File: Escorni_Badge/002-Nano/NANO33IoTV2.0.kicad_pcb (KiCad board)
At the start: 4 copper layers, 99.5 x 97.2 mm, 1 part

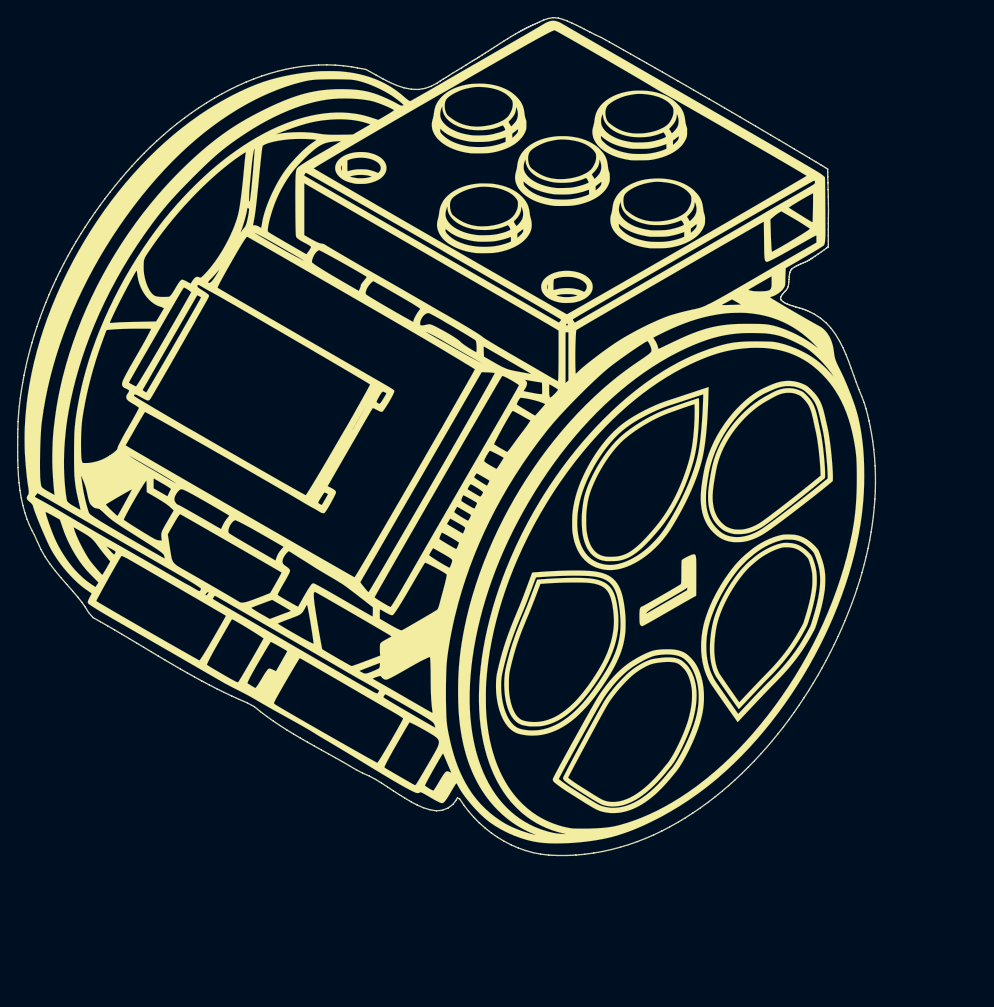
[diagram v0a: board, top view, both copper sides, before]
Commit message: Add some minors changes
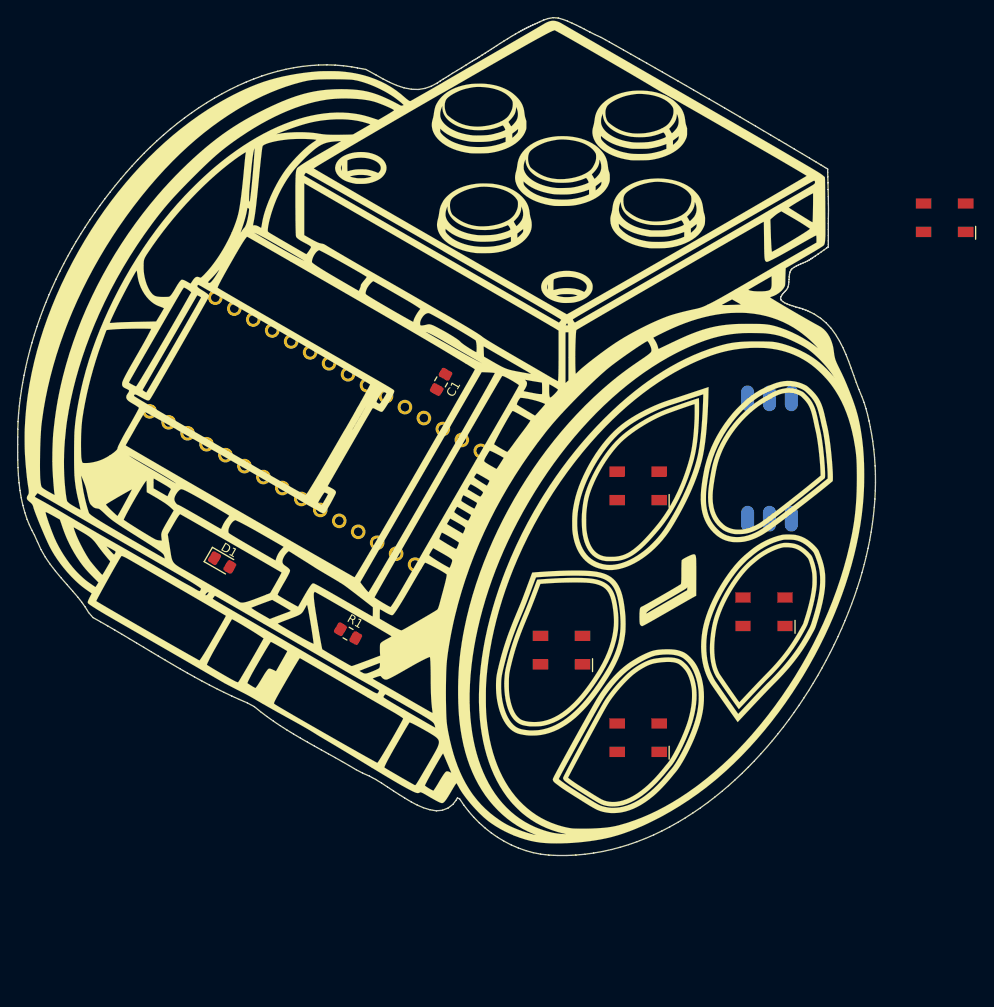
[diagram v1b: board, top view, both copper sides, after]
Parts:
- added C1: 22nF, Capacitor_SMD:C_0805_2012Metric_Pad1.15x1.40mm_HandSolder, F.Cu at (142.9, 97.8)
- added D1: LED, LED_SMD:LED_0805_2012Metric_Pad1.15x1.40mm_HandSolder, F.Cu at (117.5, 118.7)
- added J1: Arduino-NANO-33, Arduino:NANO_33_Single_Socket, F.Cu at (128.3, 103.5)
- added LED1: WS2812B, 002:WS2812B, F.Cu at (165.7, 109.9)
- added LED2: WS2812B, 002:WS2812B, F.Cu at (156.8, 128.9)
- added LED3: WS2812B, 002:WS2812B, F.Cu at (165.7, 139.1)
- added LED4: WS2812B, 002:WS2812B, F.Cu at (180.3, 124.5)
- added LED5: WS2812B, 002:WS2812B, F.Cu at (201.3, 78.7)
- added R1: 1k, Resistor_SMD:R_0805_2012Metric_Pad1.15x1.40mm_HandSolder, F.Cu at (132.1, 127.0)
- added REF**: WS2812B_Module, 002-Nano:WS2812B_Module, B.Cu at (181.0, 106.7)

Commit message: Updates
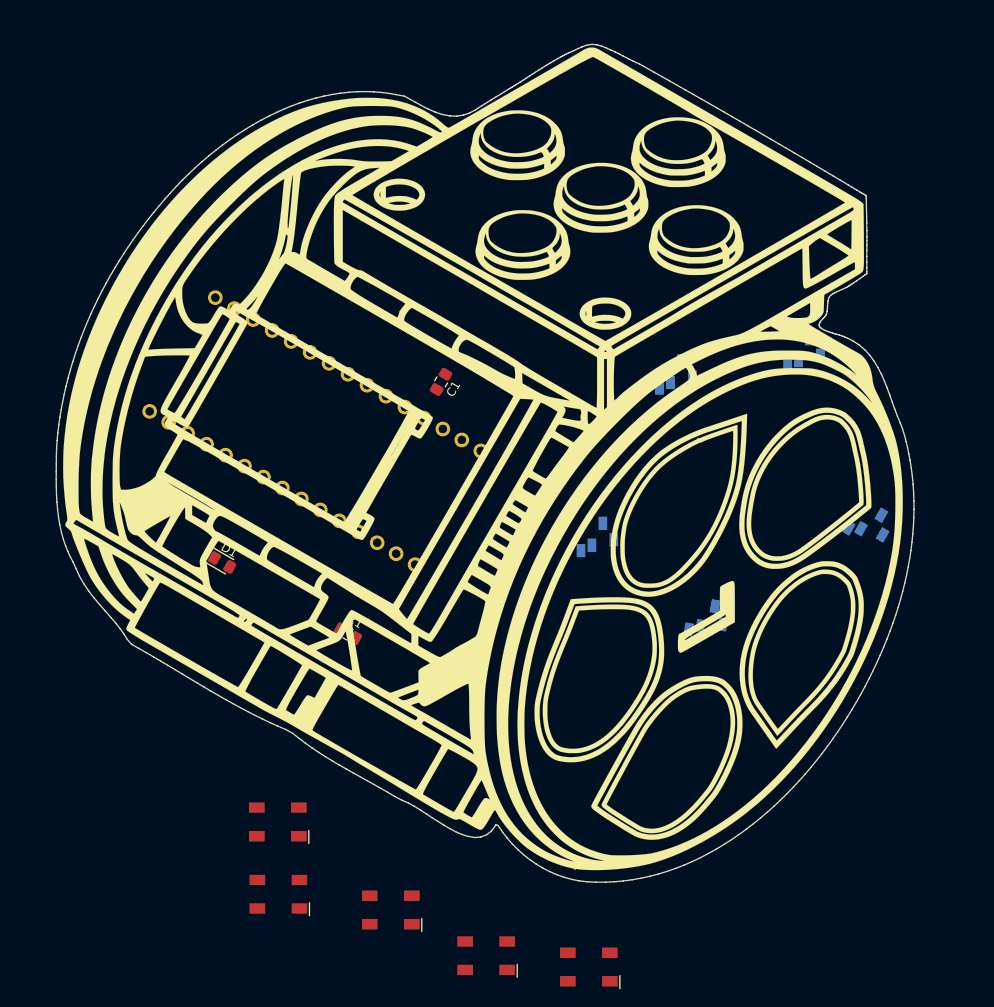
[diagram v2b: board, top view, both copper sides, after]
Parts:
- removed the REF** at (181.0, 106.7)
- removed SilKs1: Escorni_Art, 002-Nano:escorni-badge-new_05_Nano_100mm
- added REF**: P9823_Reverse_Mount_Short_Pin, 002-Nano:P9823_Reverse_Mount_Short_Pin, B.Cu at (172.6, 131.9)
- added REF**: P9823_Reverse_Mount_Short_Pin, 002-Nano:P9823_Reverse_Mount_Short_Pin, B.Cu at (189.3, 120.1)
- added REF**: P9823_Reverse_Mount_Short_Pin, 002-Nano:P9823_Reverse_Mount_Short_Pin, B.Cu at (161.0, 122.5)
- added REF**: P9823_Reverse_Mount_Short_Pin, 002-Nano:P9823_Reverse_Mount_Short_Pin, B.Cu at (170.1, 103.6)
- added REF**: P9823_Reverse_Mount_Short_Pin, 002-Nano:P9823_Reverse_Mount_Short_Pin, B.Cu at (185.0, 101.0)
- added Ref**: Val**, 002-Nano:escorni-badge-new_06_Nano_100mm, F.Cu at (148.0, 107.2)
- moved LED5 96.2 mm to (160.0, 165.7)
- moved LED1 57.2 mm to (123.9, 148.8)
- moved LED4 51.3 mm to (148.1, 164.4)
- moved LED2 43.4 mm to (124.0, 157.2)
- moved LED3 35.0 mm to (137.0, 159.1)
